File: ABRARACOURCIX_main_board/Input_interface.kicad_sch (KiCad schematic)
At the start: 12 parts, among them J4 Conn_01x04_Socket, J5 Conn_01x05_Socket, J6 Conn_01x04_Socket, J7 Conn_01x04_Socket

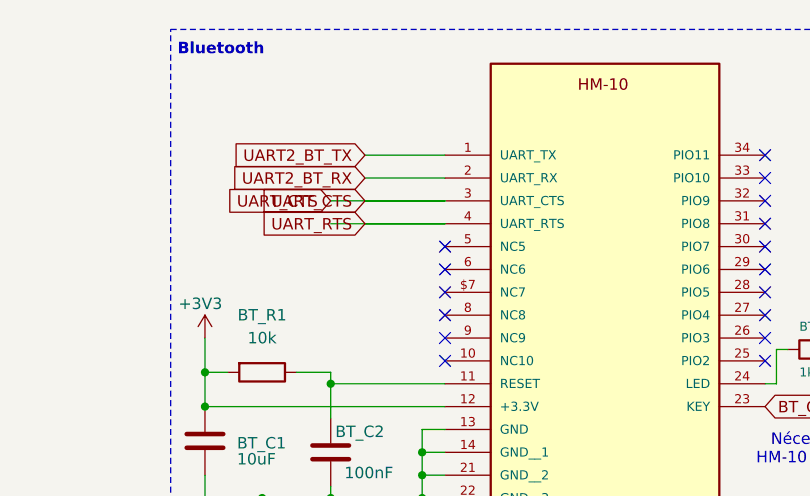
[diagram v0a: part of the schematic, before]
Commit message: Damn j'ai oublié de push y'a 2 semaines
je sais plus
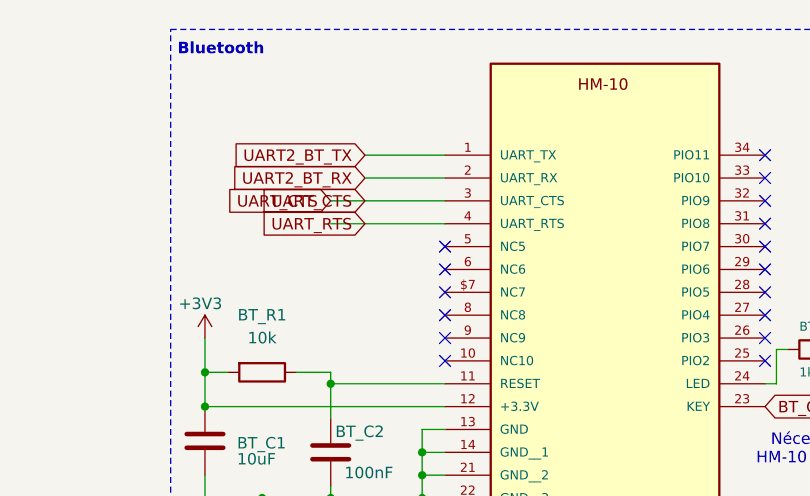
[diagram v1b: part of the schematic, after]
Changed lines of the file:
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@@
-	(wire
-		(pts
-			(xy 161.29 39.37) (xy 170.18 39.37)
-		)
-		(stroke
-			(width 0)
-			(type default)
-		)
-	)
 	(wire
 		(pts
@@
 		)
 		(stroke
-			(width 0)
-			(type default)
-		)
-	)
-	(wire
-		(pts
-			(xy 161.29 41.91) (xy 170.18 41.91)
-		)
-		(stroke
